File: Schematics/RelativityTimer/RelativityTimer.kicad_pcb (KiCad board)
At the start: 2 copper layers, 11 parts, among them J1 Conn_01x12_Female, SW1 SW_Push, SW2 SW_Push, SW3 SW_Push

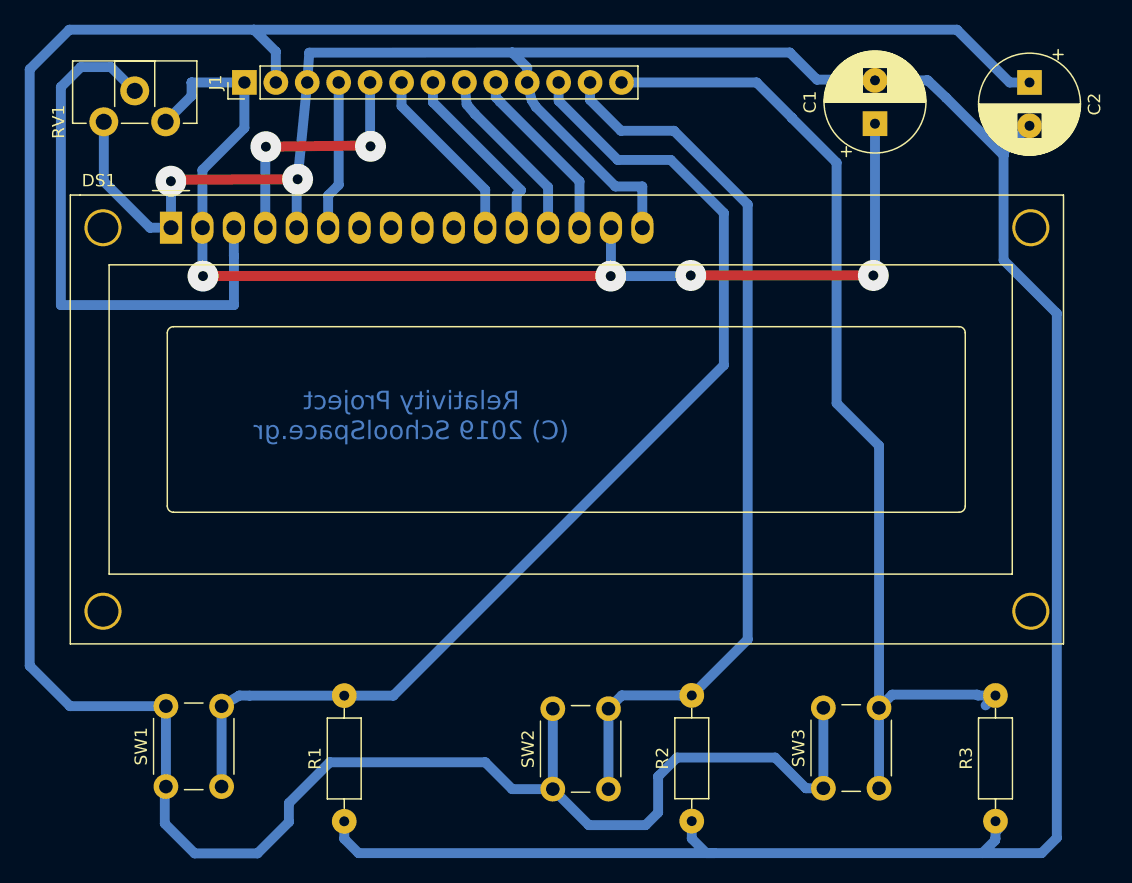
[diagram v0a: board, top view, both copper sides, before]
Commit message: Minor changes to 1.0 printed board
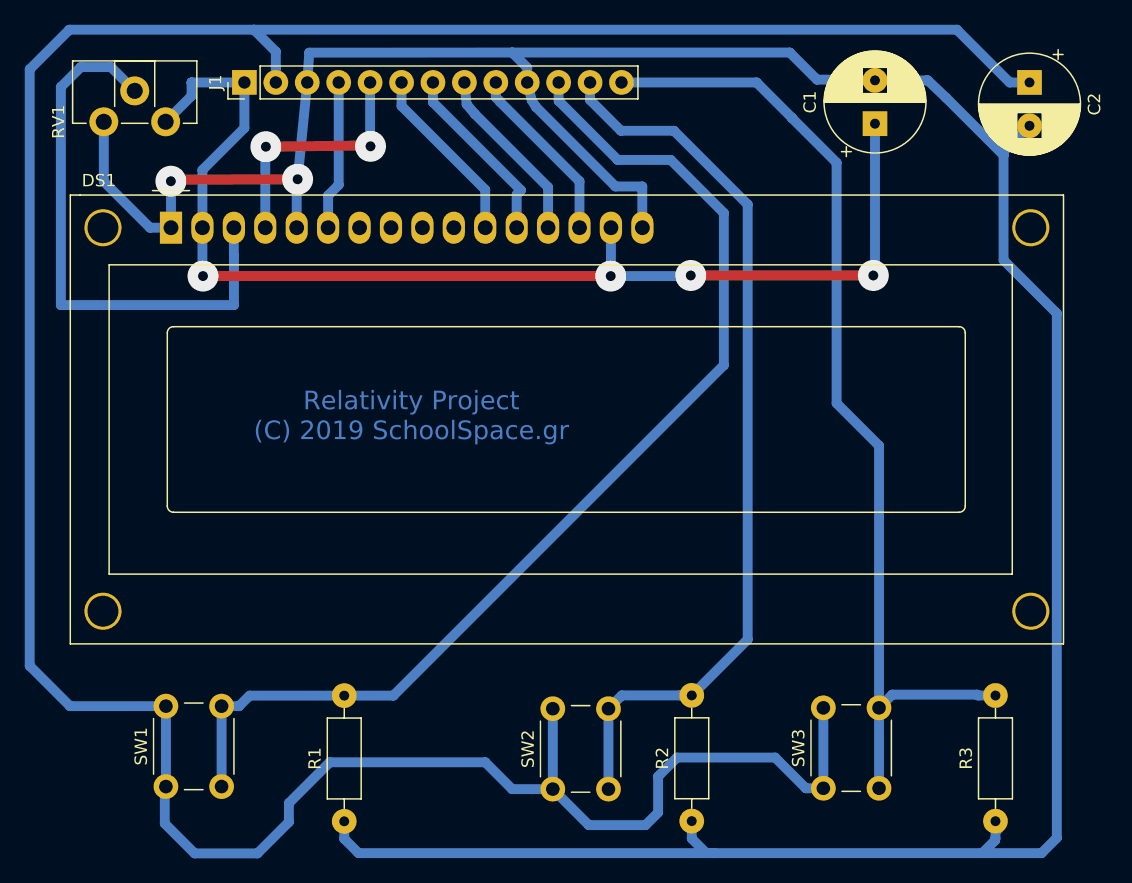
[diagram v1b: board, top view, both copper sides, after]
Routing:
- net Net-(J1-Pad13): track 83.1 -> 82.0 mm
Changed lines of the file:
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@@
     (thickness 1.6)
     (drawings 1)
-    (tracks 175)
+    (tracks 174)
     (zones 0)
     (modules 11)
@@
     (visible_elements 7FFFFFFF)
     (pcbplotparams
-      (layerselection 0x010fc_ffffffff)
+      (layerselection 0x00000_fffffffe)
       (usegerberextensions false)
       (usegerberattributes false)
@@
       (padsonsilk false)
       (subtractmaskfromsilk false)
-      (outputformat 1)
-      (mirror false)
+      (outputformat 4)
+      (mirror true)
       (drillshape 1)
       (scaleselection 1)
-      (outputdirectory ""))
+      (outputdirectory "D:/Data/Desktop/"))
   )
   (net 0 "")
@@
   )
   (gr_text "Relativity Project\n(C) 2019 SchoolSpace.gr" (at 112.13084 62.01918) (layer B.Cu)
-    (effects (font (size 1.5 1.5) (thickness 0.3)) (justify mirror))
+    (effects (font (size 1.5 1.5) (thickness 0.3)))
   )
   (segment (start 121.49836 33.890559) (end 120.2817 32.673899) (width 0.8) (layer B.Cu) (net 1))
@@
   (segment (start 96.79344 92.00642) (end 96.79344 85.50642) (width 0.8) (layer B.Cu) (net 2) (status 30))
   (segment (start 99.058413 84.65566) (end 106.70794 84.65566) (width 0.8) (layer B.Cu) (net 2) (status 20))
-  (segment (start 96.79344 85.50642) (end 98.22942 84.64804) (width 0.8) (layer B.Cu) (net 2) (status 10))
-  (segment (start 98.22942 84.64804) (end 99.058413 84.65566) (width 0.8) (layer B.Cu) (net 2))
   (segment (start 124.03836 36.57854) (end 124.03836 35.09264) (width 0.8) (layer B.Cu) (net 2) (status 20))
   (segment (start 110.6805 84.65566) (end 137.39114 57.94502) (width 0.8) (layer B.Cu) (net 2))
@@
   (segment (start 133.10362 41.35628) (end 128.8161 41.35628) (width 0.8) (layer B.Cu) (net 2))
   (segment (start 128.8161 41.35628) (end 124.03836 36.57854) (width 0.8) (layer B.Cu) (net 2))
+  (segment (start 98.207653 85.50642) (end 96.79344 85.50642) (width 0.8) (layer B.Cu) (net 2))
+  (segment (start 99.058413 84.65566) (end 98.207653 85.50642) (width 0.8) (layer B.Cu) (net 2))
   (segment (start 128.06592 92.21216) (end 128.06592 85.71216) (width 0.8) (layer B.Cu) (net 3) (status 30))
   (segment (start 129.1402 84.63788) (end 128.06592 85.71216) (width 0.8) (layer B.Cu) (net 3) (status 20))
@@
   (segment (start 126.57836 35.09264) (end 126.57836 36.506853) (width 0.8) (layer B.Cu) (net 3))
   (segment (start 126.57836 36.506853) (end 129.0701 38.998593) (width 0.8) (layer B.Cu) (net 3))
-  (segment (start 159.3469 84.6455) (end 158.546901 85.445499) (width 0.8) (layer B.Cu) (net 4) (status 30))
   (segment (start 157.932687 84.6455) (end 157.861567 84.57438) (width 0.8) (layer B.Cu) (net 4))
   (segment (start 159.3469 84.6455) (end 157.932687 84.6455) (width 0.8) (layer B.Cu) (net 4) (status 10))
